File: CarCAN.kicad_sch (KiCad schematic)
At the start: 17 parts, among them IC1 TCAN337DCNR, J6 CarCANConnector, J8 CarCANConnector, U13 CDSOT23-T24CAN, U14 MCP2515-E/STVAO, Y4 8 MHz

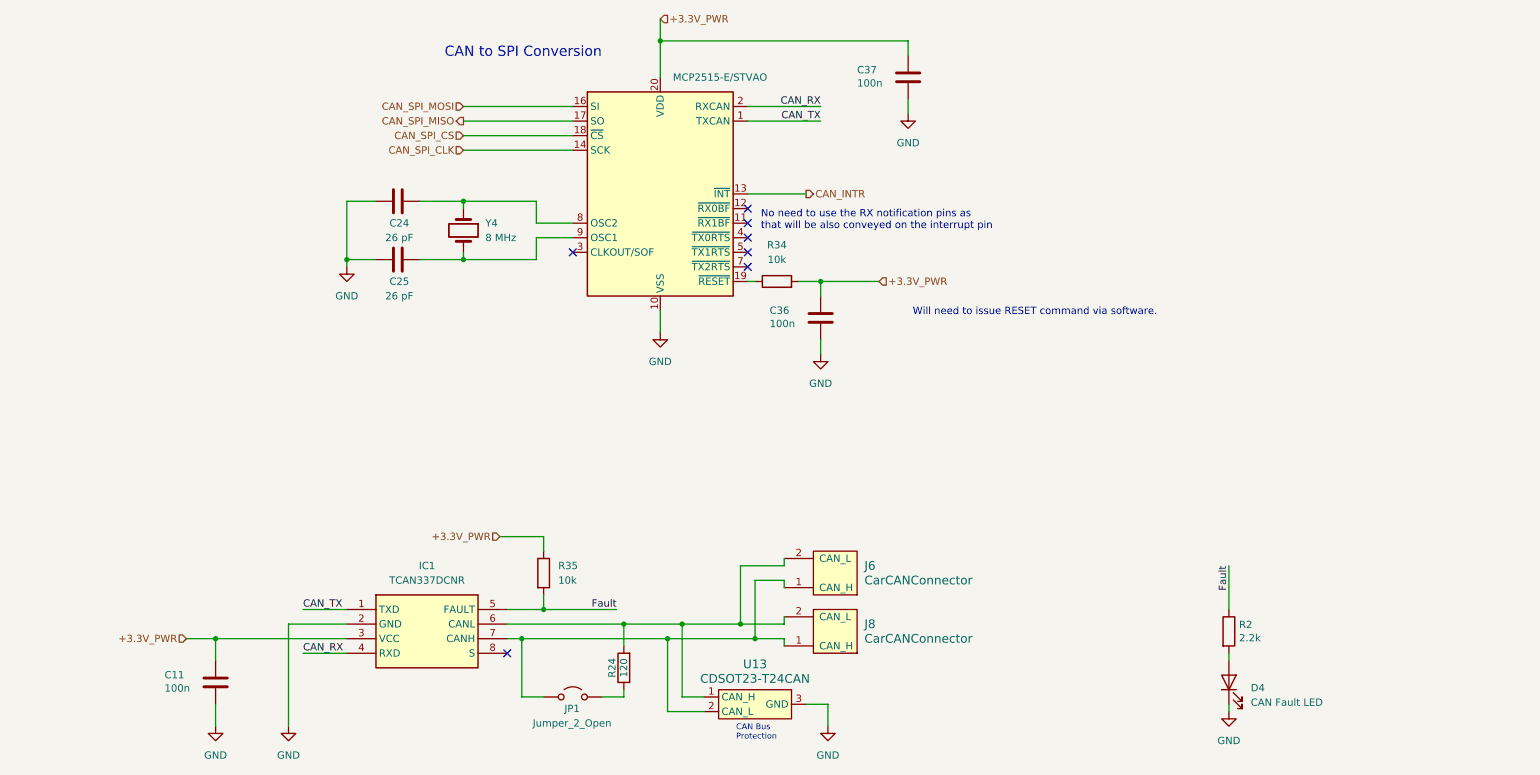
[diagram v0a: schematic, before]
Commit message: my life is horrible
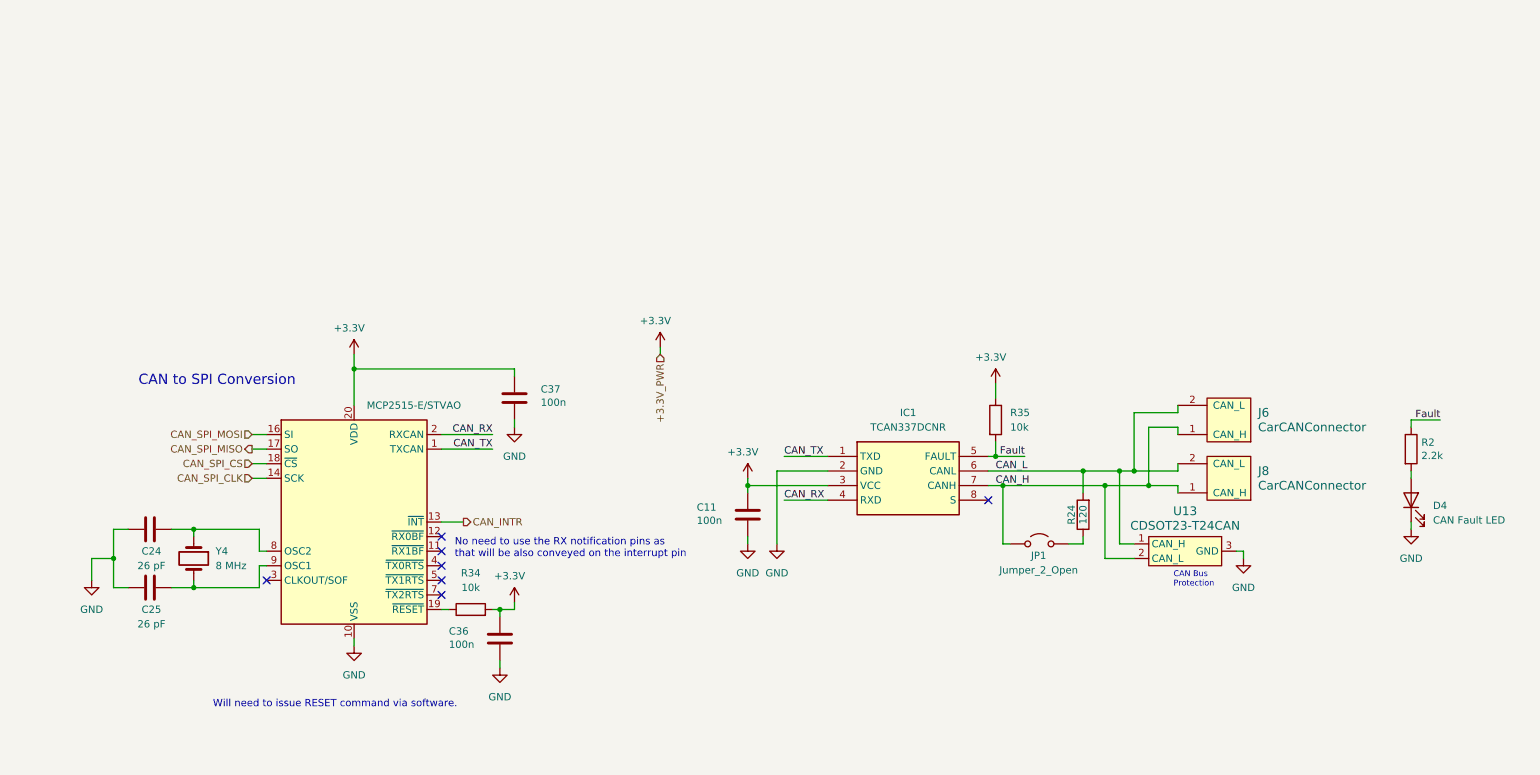
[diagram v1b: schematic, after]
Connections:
- net CAN_L: now reaches IC1.6 (CANL), J6.2 (CAN_L), J8.2 (CAN_L), R24.2, U13.1 (CAN_H)
- net CAN_H: now reaches IC1.7 (CANH), J6.1 (CAN_H), J8.1 (CAN_H), JP1.1 (A), U13.2 (CAN_L)
- net +3.3V_PWR renamed +3.3V
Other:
- moved on the sheet: C11, C24, C25, C36, C37, D4, IC1, J6, J8, JP1, R2, R24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

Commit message: Schem done? [plz full review], redoing layout
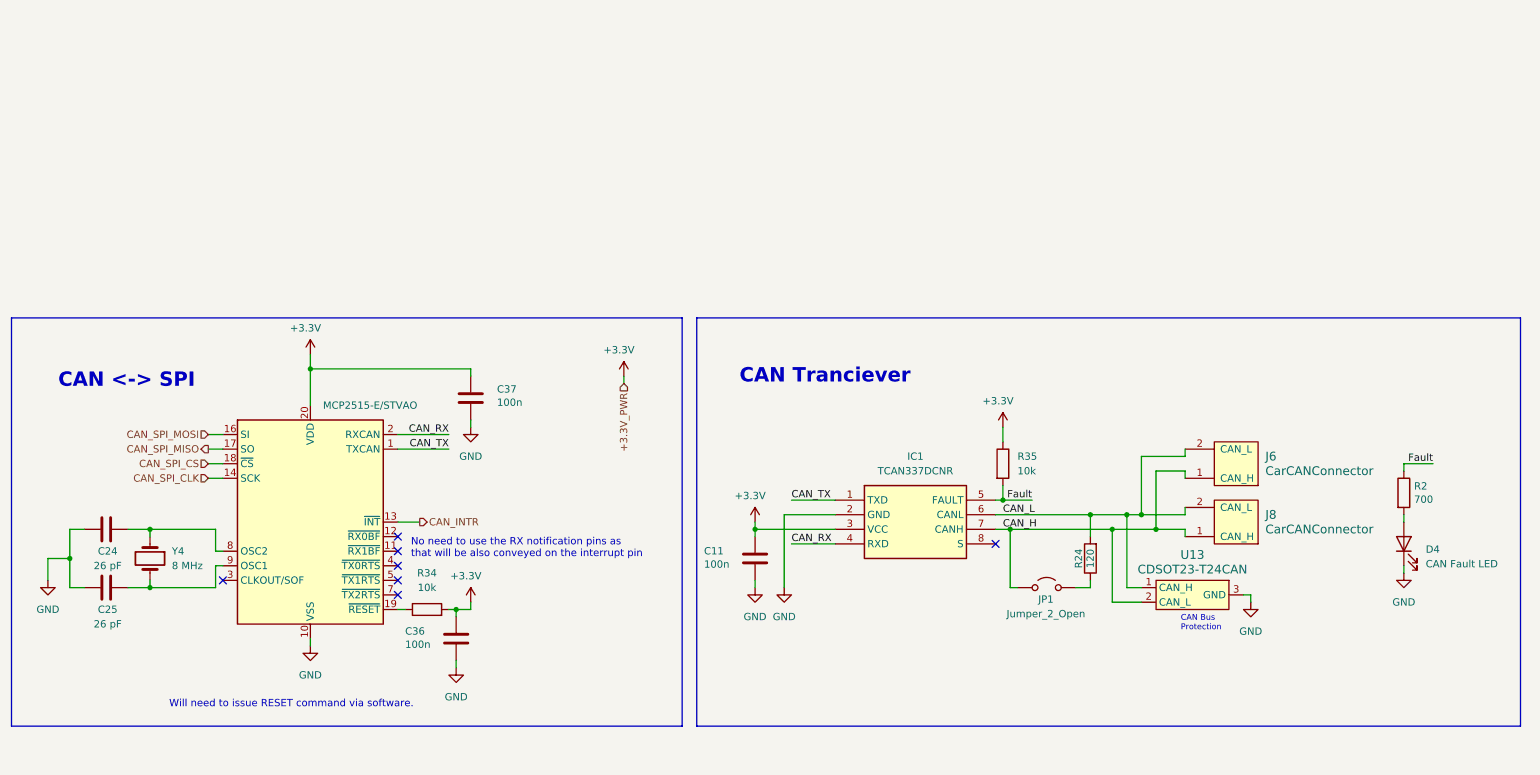
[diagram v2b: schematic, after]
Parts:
- R2: value 2.2k -> 700
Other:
- note added: "CAN <-> SPI"
- note added: "CAN Tranciever"
- note removed: "CAN to SPI Conversion"
- moved on the sheet: C11, C24, C25, C36, C37, D4, IC1, J6, J8, JP1, R2, R24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
